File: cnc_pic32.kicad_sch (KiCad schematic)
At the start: 0 parts

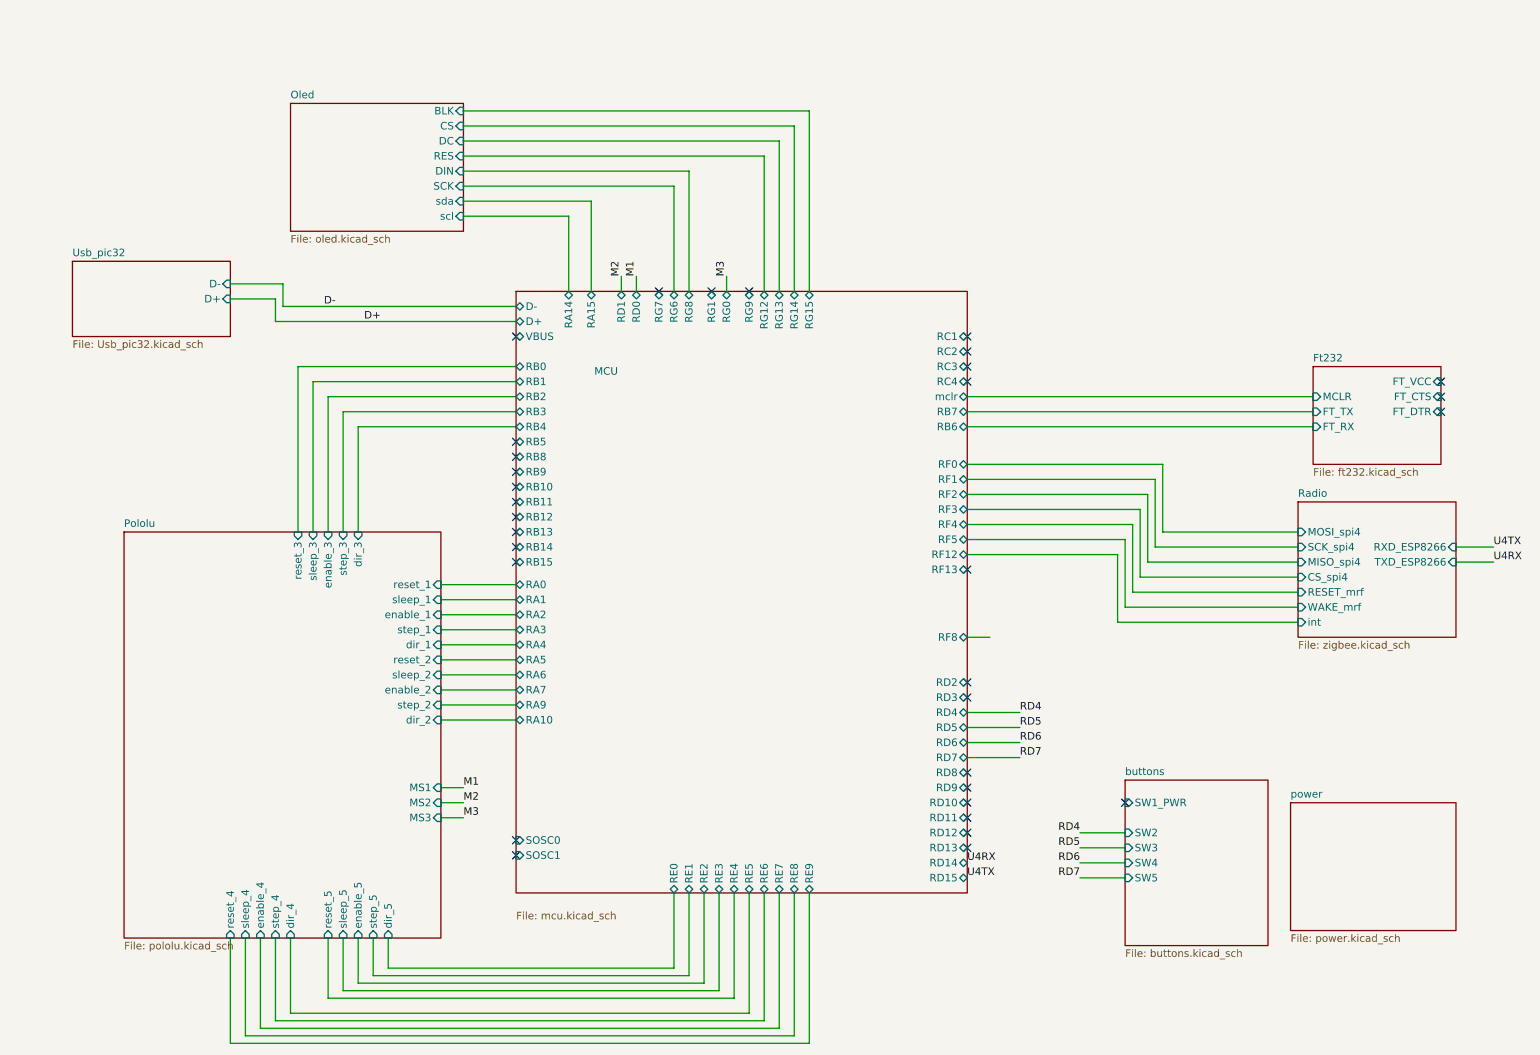
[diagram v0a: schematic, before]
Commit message: updated
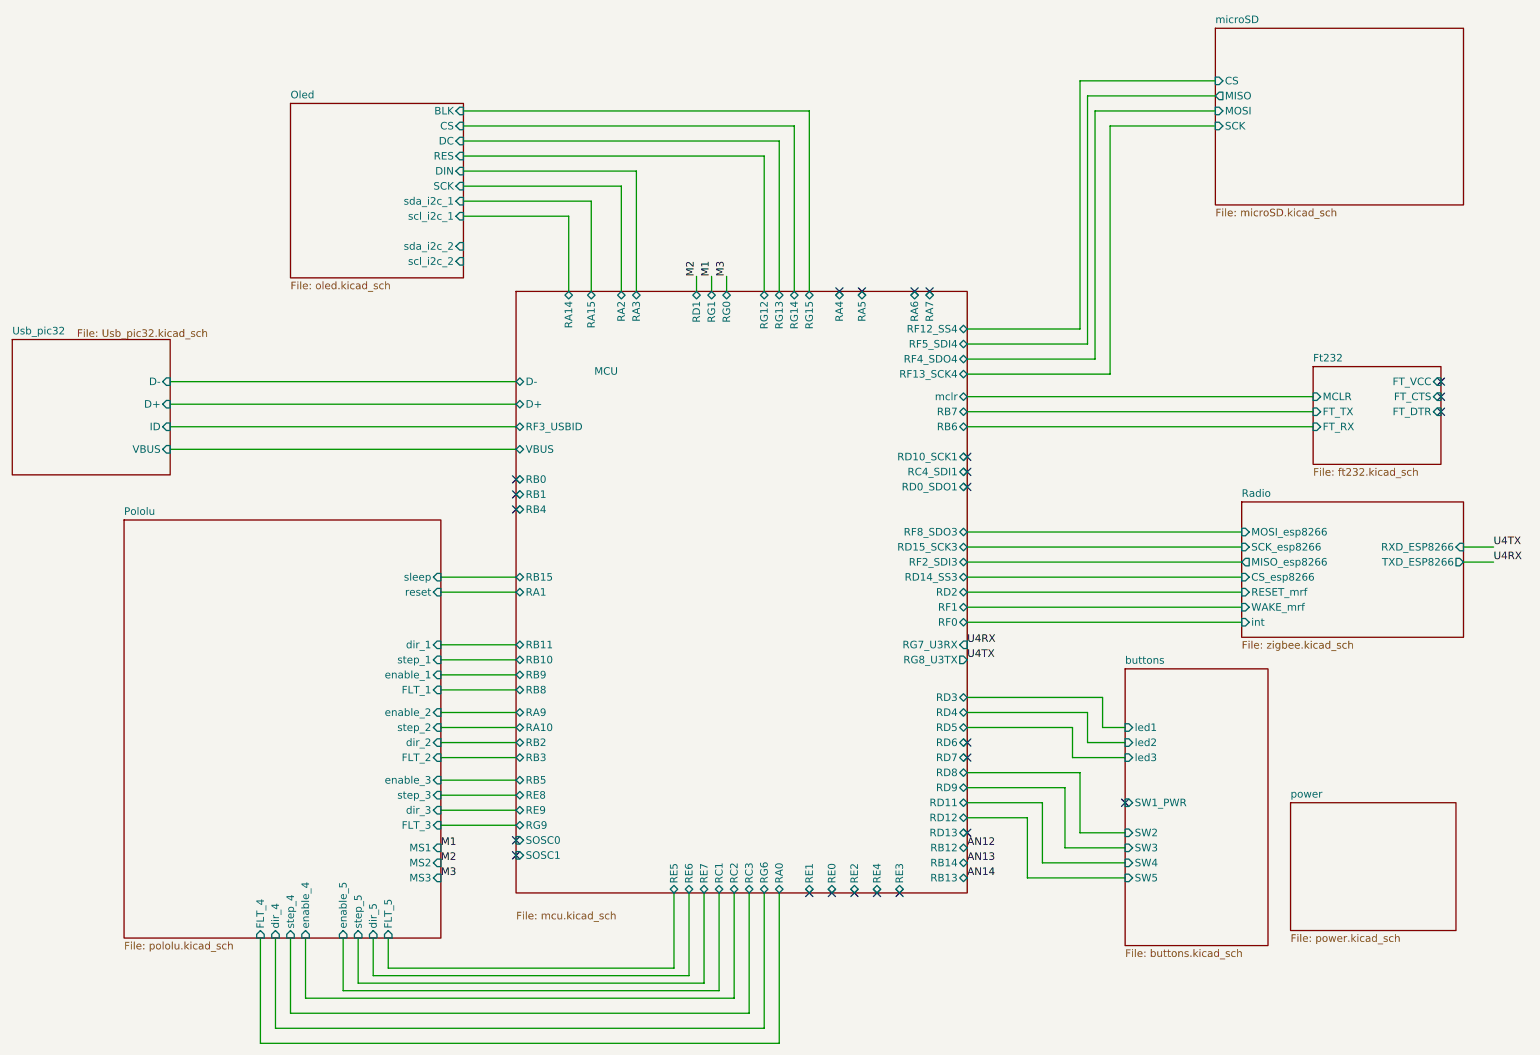
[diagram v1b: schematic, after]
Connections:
- no-connect marks 32 -> 24
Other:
- added sheet microSD (microSD.kicad_sch)
- sheet MCU ports: added RC4_SDI1, RD0_SDO1, RD10_SCK1, RD14_SS3, RD15_SCK3, RF12_SS4, RF13_SCK4, RF2_SDI3, RF3_USBID, RF4_SDO4, RF5_SDI4, RF8_SDO3, RG7_U3RX, RG8_U3TX; removed RC4, RD0, RD10, RD14, RD15, RF12, RF13, RF2, RF3, RF4, RF5, RF8, RG7, RG8
- sheet Oled ports: added scl_i2c_1, scl_i2c_2, sda_i2c_1, sda_i2c_2; removed scl, sda
- sheet Pololu ports: added FLT_1, FLT_2, FLT_3, FLT_4, FLT_5, reset, sleep; removed reset_1, reset_2, reset_3, reset_4, reset_5, sleep_1, sleep_2, sleep_3, sleep_4, sleep_5
- sheet Radio ports: added CS_esp8266, MISO_esp8266, MOSI_esp8266, SCK_esp8266; removed CS_spi4, MISO_spi4, MOSI_spi4, SCK_spi4
- sheet Usb_pic32 ports: added ID, VBUS; removed none
- sheet buttons ports: added led1, led2, led3; removed none
